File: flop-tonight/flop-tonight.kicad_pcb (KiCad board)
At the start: 2 copper layers, 23 parts, among them J1 Bus_ISA_8bit, J2 Conn_02x17_Odd_Even, U1 PC8477BV, U2 74ALS138, U3 74ALS138, Y1 24 MHz

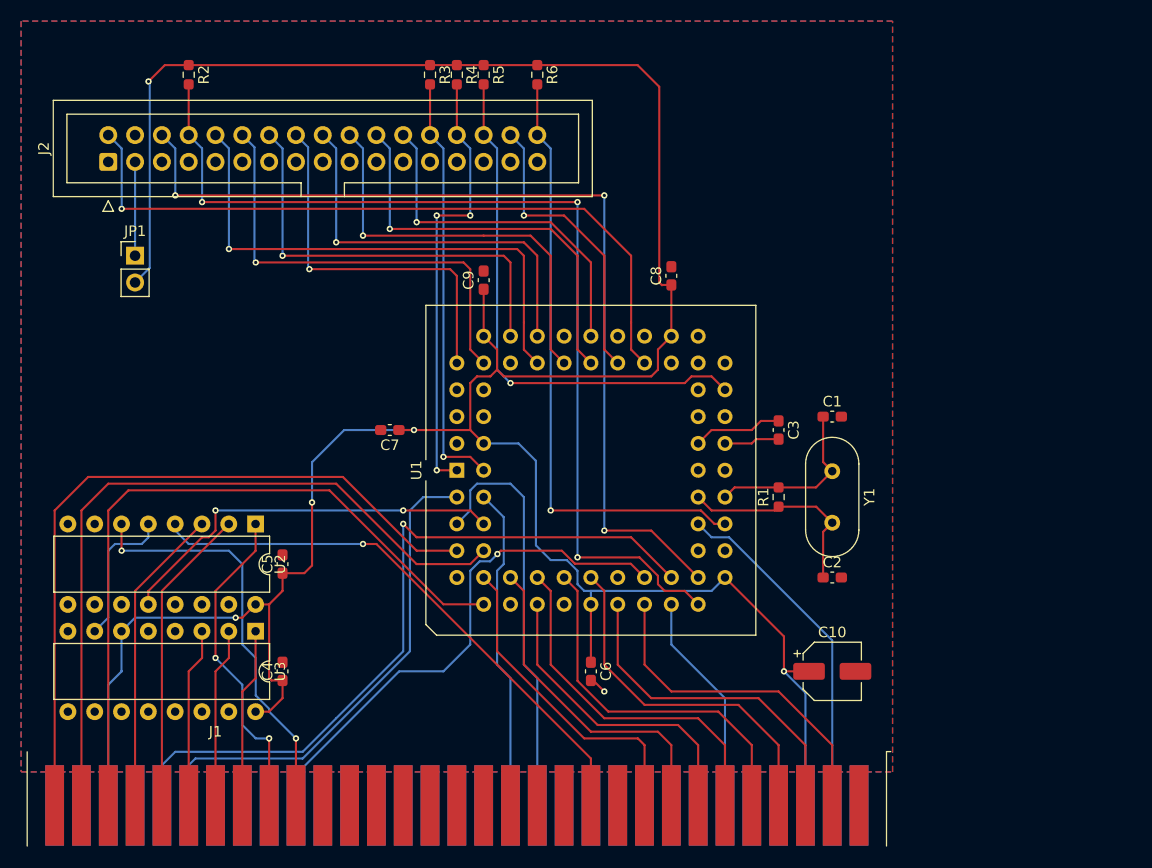
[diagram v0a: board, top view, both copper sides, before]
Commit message: Adding flop-tonight updates
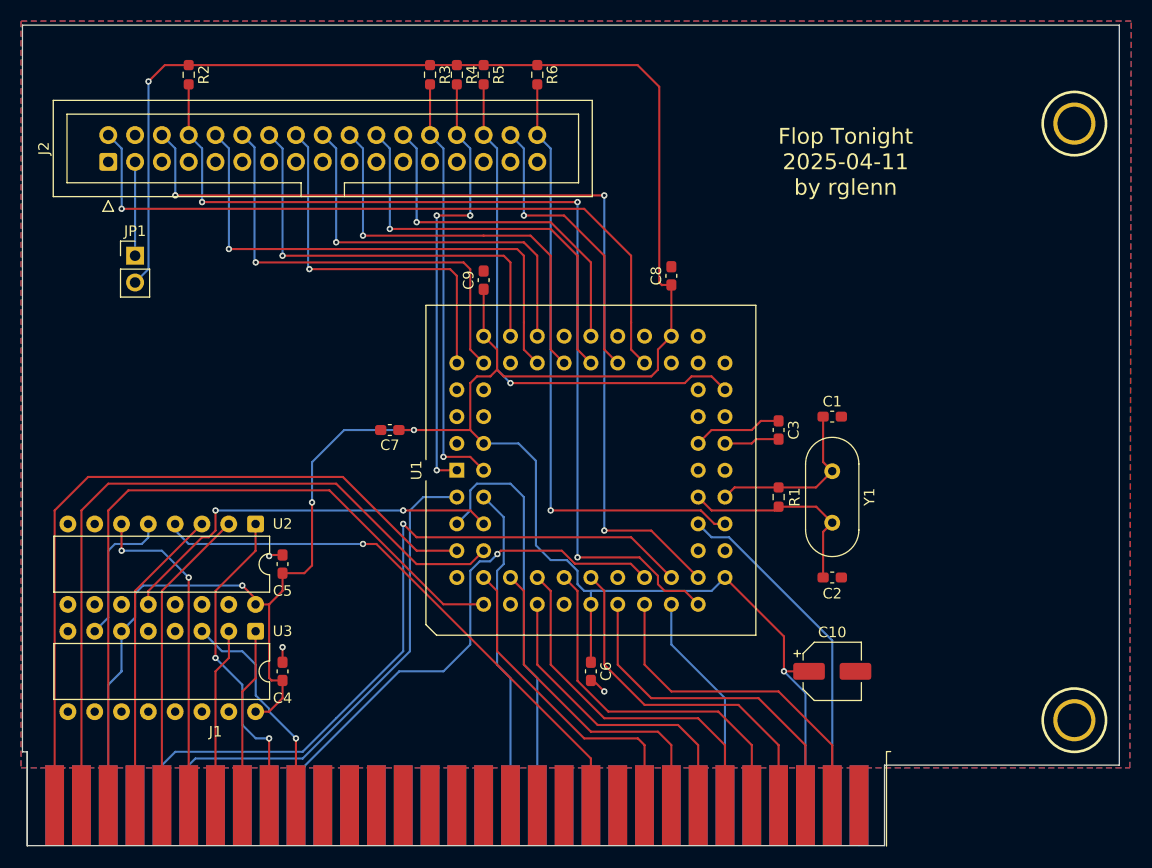
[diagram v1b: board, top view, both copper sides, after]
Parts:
- added BRACKET1: ~, pc-parts:PC_BRACKET_ISA_KEYSTONE_9202_Rev1, F.Cu at (152.4, 130.8)
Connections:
- U2 pad 6: /A9 -> /A5
- U3 pad 3: /A5 -> /A9
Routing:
- net /A9: track 39.5 -> 21.3 mm, vias 2 -> 1
- net /A5: track 17.0 -> 31.5 mm, vias 0 -> 2
- net +5V: track 280.1 -> 283.1 mm
- net GND: track 1.70 -> 4.44 mm, vias 1 -> 3
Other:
- board outline added: 103.9 x 77.7 mm
- board text added: "Flop Tonight 2025-04-11 by rglenn"
